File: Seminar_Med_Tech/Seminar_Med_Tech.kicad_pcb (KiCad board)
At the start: 2 copper layers, 96 x 88 mm, 160 parts, among them J1 CONN_02X08, J3 CONN_02X10, J5 CONN_02X10, J7 CONN_02X08, U1 OPA132, U18 ADS1298, U20 ADS1298, U4 LM317T, U5 LM317T, U6 LM337K

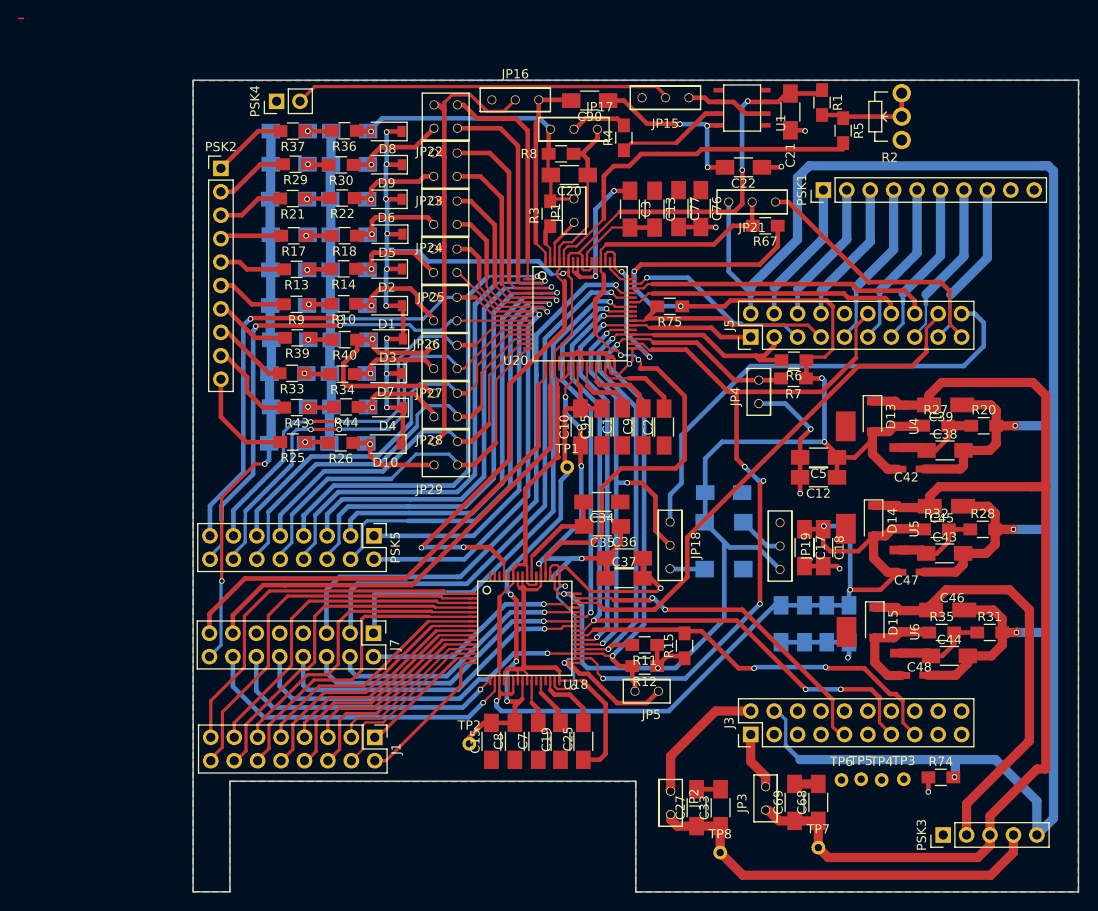
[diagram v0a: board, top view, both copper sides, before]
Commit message: Update
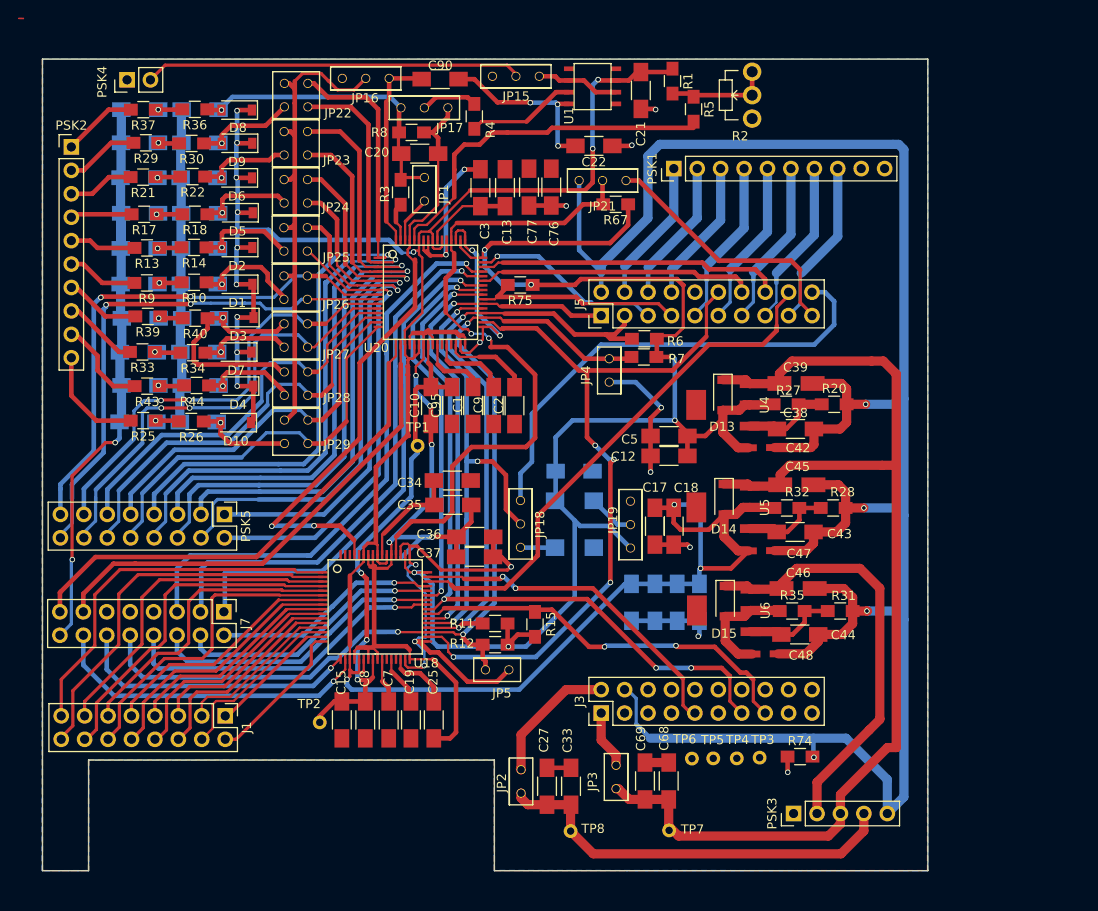
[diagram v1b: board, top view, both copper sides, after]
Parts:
- moved C12 16.4 mm to (143.8, 95.7)
- moved C13 16.4 mm to (126.0, 66.6)
- moved C14 16.4 mm to (147.1, 111.6)
- moved C16 16.4 mm to (142.3, 111.6)
- moved C17 16.4 mm to (142.3, 103.3)
- moved C21 16.4 mm to (140.8, 56.1)
- moved C25 16.4 mm to (118.3, 124.3)
- moved C3 16.4 mm to (123.4, 66.6)
- moved C35 16.4 mm to (120.4, 101.0)
- moved C39 16.4 mm to (157.1, 88.7)
- moved C44 16.4 mm to (158.0, 115.1)
- moved C48 16.4 mm to (154.7, 116.8)
- moved C5 16.4 mm to (143.8, 93.6)
- moved D14 16.4 mm to (149.8, 100.4)
- moved D15 16.4 mm to (149.9, 111.5)
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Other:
- outline, holes or cut-outs redrawn
